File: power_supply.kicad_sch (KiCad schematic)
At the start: 40 parts, among them J1 USB_C_Receptacle_USB2.0_16P, J2 B2B-XH-A, J3 USB_C_Receptacle_USB2.0_16P, SW1 SW_SPDT

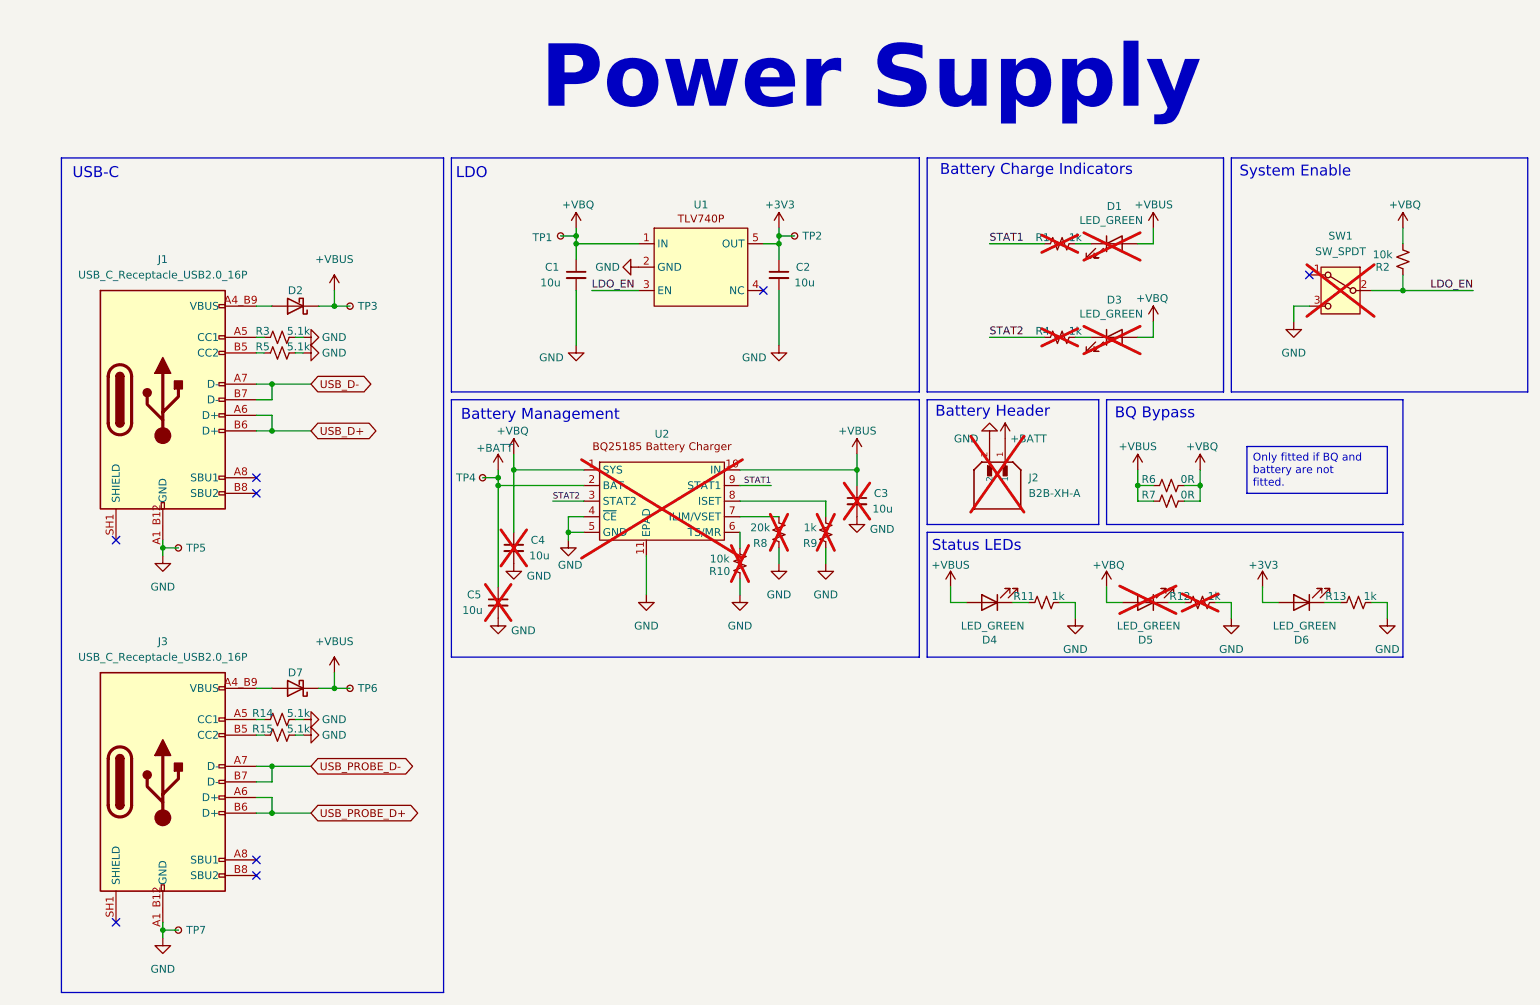
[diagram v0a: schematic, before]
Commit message: wip: adds more routing
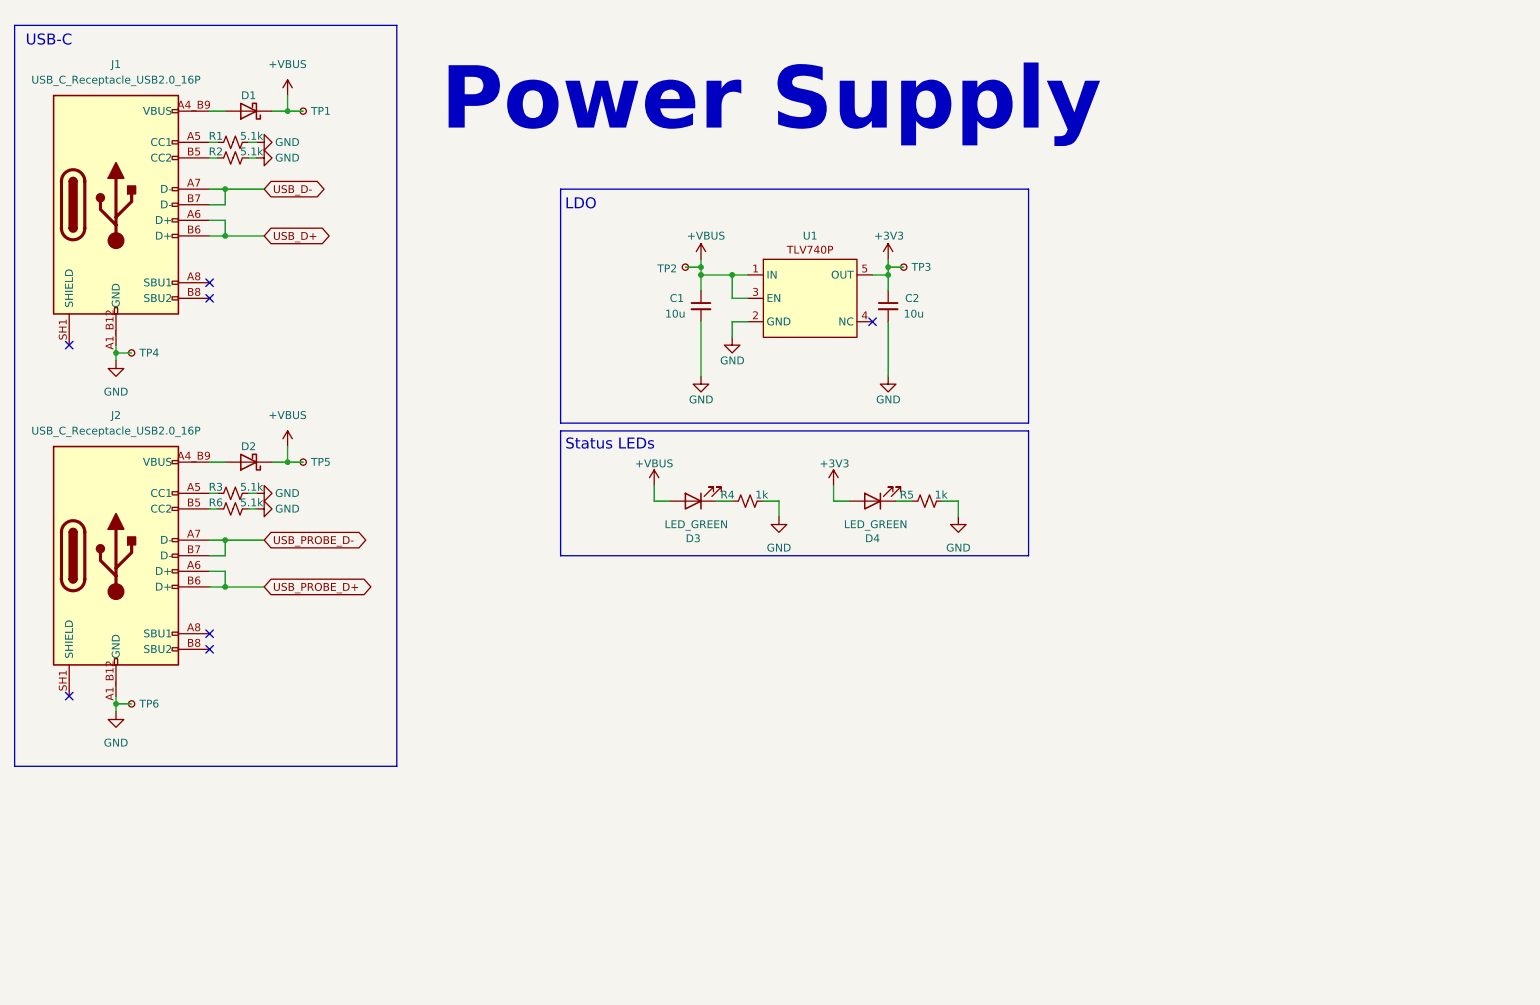
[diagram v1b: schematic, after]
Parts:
- removed C3, C4, C5: 10u, Capacitor_SMD:C_0805_2012Metric, symbol Device:C_Small
- removed D1, D3, D5: LED_GREEN, LED_SMD:LED_0603_1608Metric, symbol Device:LED
- removed J2: B2B-XH-A, B2B-XH-A:JST_B2B-XH-A, symbol B2B-XH-A:B2B-XH-A
- removed R1, R12, R4, R9: 1k, Resistor_SMD:R_0402_1005Metric, symbol Device:R_Small_US
- removed R10, R2: 10k, Resistor_SMD:R_0402_1005Metric, symbol Device:R_Small_US
- removed R6, R7: 0R, Resistor_SMD:R_1206_3216Metric, symbol Device:R_Small_US
- removed R8: 20k, Resistor_SMD:R_0402_1005Metric, symbol Device:R_Small_US
- removed SW1: SW_SPDT, power_supply:SW_SLW-121456-3A-N-D, symbol Switch:SW_SPDT
- removed TP4: TestPoint_Small, TestPoint:TestPoint_Pad_D1.0mm, symbol Connector:TestPoint_Small
- removed U2: ~, power_supply:WSON10_DLH_TEX, symbol Power_PMIC_TexasInstruments_BQ25185:BQ25185DLHR
- renumbered D2 to D1, D7 to D2, D4 to D3, D6 to D4, J3 to J2, R3 to R1, R5 to R2, R14 to R3, R11 to R4, R13 to R5, R15 to R6, TP3 to TP1, TP1 to TP2, TP2 to TP3, TP5 to TP4, TP6 to TP5, TP7 to TP6
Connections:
- net +VBQ is gone; now on net +VBUS: C1.1, TP2.1, U1.1 (IN)
- net LDO_EN is gone; now on net +VBUS: U1.3 (EN)
- no-connect marks 8 -> 7
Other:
- note removed: "BQ Bypass"
- note removed: "Battery Charge Indicators"
- note removed: "Battery Header"
- note removed: "Battery Management"
- note removed: "System Enable"
- moved on the sheet: C1, C2, D1, D2, D3, D4, J1, J2, R1, R2, R3, R4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
